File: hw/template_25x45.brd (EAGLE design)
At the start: 25 x 45 mm, 23 parts, among them J1 GROVE-4P-2.0-3470130P1, J2 GROVE-4P-2.0-3470130P1

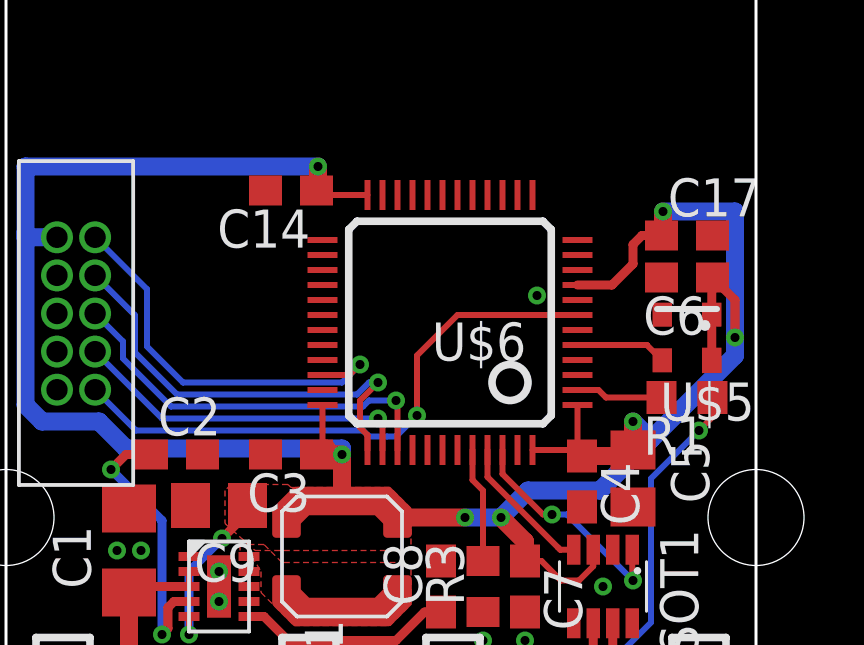
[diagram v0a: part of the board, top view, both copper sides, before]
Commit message: updated to STM32F303 family
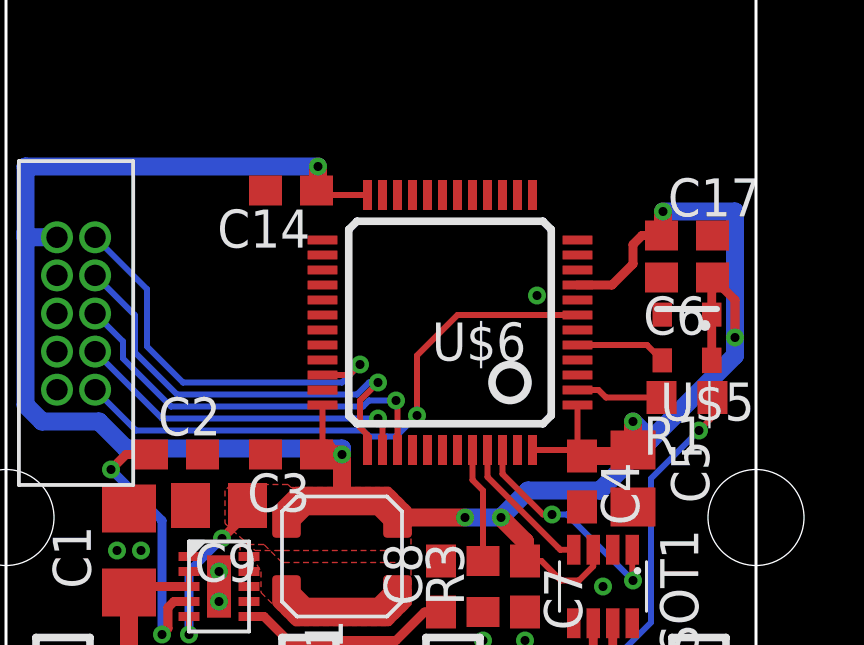
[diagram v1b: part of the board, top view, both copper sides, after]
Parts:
- U$6: value STM32F103CX -> STM32F303C
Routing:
- net +3V3: track 86.0 -> 86.7 mm
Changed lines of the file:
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@@
 <element name="U$3" library="maxim" package="TDFN-10" value="MAX17501" x="7.1" y="7.7"/>
 <element name="J1" library="OPL Eagle Library" package="4P-2.0" value="GROVE-4P-2.0-3470130P1" x="6" y="3.2" rot="R180"/>
-<element name="U$6" library="st" package="LQFP48" value="STM32F103CX" x="14.8" y="16.5" rot="R180"/>
+<element name="U$6" library="st" package="LQFP48" value="STM32F303C" x="14.8" y="16.5" rot="R180"/>
 <element name="SOT1" library="maxim" package="SOT23-8L" value="MAX3051EKA" x="19.9" y="7.7" rot="R180"/>
 <element name="U$1" library="r2p_pcb" package="25X45" value="PCB_25X45" x="0" y="0"/>
@@
 <contactref element="J1" pad="4"/>
 <contactref element="J2" pad="4"/>
+<contactref element="U$6" pad="47"/>
 <contactref element="U$6" pad="23"/>
 <contactref element="U$6" pad="35"/>
-<contactref element="U$6" pad="47"/>
 <contactref element="U$6" pad="8"/>
 <polygon width="0.2" layer="16" thermals="no">
@@
 <contactref element="U$3" pad="P$5"/>
 <contactref element="U$6" pad="9"/>
+<contactref element="U$6" pad="48"/>
 <contactref element="U$6" pad="24"/>
 <contactref element="U$6" pad="36"/>
-<contactref element="U$6" pad="48"/>
 <contactref element="U$6" pad="1"/>
 <via x="6.1" y="6.1" extent="1-16" drill="0.3"/>
@@
 <wire x1="17.3" y1="8.55" x2="17.85" y2="8.55" width="0.2" layer="1"/>
 <wire x1="17.85" y1="8.55" x2="18.5" y2="7.9" width="0.2" layer="1"/>
-<wire x1="10.55" y1="13.75" x2="10.55" y2="12.3" width="0.2" layer="1"/>
 <wire x1="10.55" y1="12.3" x2="10.35" y2="12.1" width="0.2" layer="1"/>
 <via x="11.2" y="12.1" extent="1-16" drill="0.3"/>
@@
 <wire x1="8.05" y1="10.75" x2="7.95" y2="10.75" width="0.3" layer="1"/>
 <wire x1="10.55" y1="12.3" x2="10.7" y2="12.3" width="0.6" layer="1"/>
-<wire x1="17.55" y1="12.25" x2="19" y2="12.25" width="0.2" layer="1"/>
 <wire x1="19" y1="12.25" x2="19.2" y2="12.05" width="0.2" layer="1"/>
 <wire x1="19.05" y1="13.75" x2="19.05" y2="12.2" width="0.2" layer="1"/>
@@
 <wire x1="10.4" y1="21.7" x2="10.4" y2="20.85" width="0.6" layer="1"/>
 <wire x1="10.4" y1="20.85" x2="10.35" y2="20.9" width="0.6" layer="1"/>
-<wire x1="12.05" y1="20.75" x2="10.5" y2="20.75" width="0.2" layer="1"/>
 <wire x1="10.5" y1="20.75" x2="10.4" y2="20.85" width="0.2" layer="1"/>
 <wire x1="10.4" y1="20.85" x2="10.35" y2="20.9" width="0.2" layer="1"/>
@@
 <wire x1="23.525" y1="16.7625" x2="23.525" y2="17.975" width="0.3" layer="1"/>
 <wire x1="23.525" y1="17.975" x2="23.55" y2="18" width="0.3" layer="1"/>
+<wire x1="17.55" y1="12.25" x2="19.2" y2="12.25" width="0.2" layer="1"/>
+<wire x1="19.2" y1="12.25" x2="19.2" y2="12.05" width="0.2" layer="1"/>
+<wire x1="12.05" y1="20.75" x2="10.35" y2="20.75" width="0.2" layer="1"/>
+<wire x1="10.35" y1="20.75" x2="10.35" y2="20.9" width="0.2" layer="1"/>
+<wire x1="10.55" y1="12.3" x2="10.55" y2="13.75" width="0.2" layer="1"/>
 </signal>
 <signal name="JTMS">

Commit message: added missing values
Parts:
- C1: value (none) -> 1u
- C9: value (none) -> 10uF
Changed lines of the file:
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@@
 <?xml version="1.0" encoding="utf-8"?>
 <!DOCTYPE eagle SYSTEM "eagle.dtd">
-<eagle version="6.4">
+<eagle version="6.6.0">
 <drawing>
 <settings>
@@
 <element name="J2" library="OPL Eagle Library" package="4P-2.0" value="GROVE-4P-2.0-3470130P1" x="19" y="3.2" rot="R180"/>
 <element name="U$2" library="coilcraft" package="LPS4018" value="LPS4018" x="11.2" y="8.7" rot="R90"/>
-<element name="C1" library="rcl" package="C1206" value="" x="4.1" y="8.9" rot="R90"/>
+<element name="C1" library="rcl" package="C1206" value="1u" x="4.1" y="8.9" rot="R90"/>
 <element name="C2" library="rcl" package="C0603" value="1u" x="5.7" y="12.1"/>
 <element name="C8" library="rcl" package="C0603" value="10n" x="14.5" y="7.7" rot="R90"/>
-<element name="C9" library="rcl" package="C0805" value="" x="7.1" y="10.4" rot="R180"/>
+<element name="C9" library="rcl" package="C0805" value="10uF" x="7.1" y="10.4" rot="R180"/>
 <element name="U$3" library="maxim" package="TDFN-10" value="MAX17501" x="7.1" y="7.7"/>
 <element name="J1" library="OPL Eagle Library" package="4P-2.0" value="GROVE-4P-2.0-3470130P1" x="6" y="3.2" rot="R180"/>
